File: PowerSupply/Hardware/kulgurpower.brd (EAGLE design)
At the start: 102 x 86.5 mm, 138 parts, among them M1 MST2V, M2 MST2V, M3 MST2V, M4 MST2V, X1 1727036, X2 2534-, X3 22-23-2031, X4 22-23-2031, X5 22-23-2021

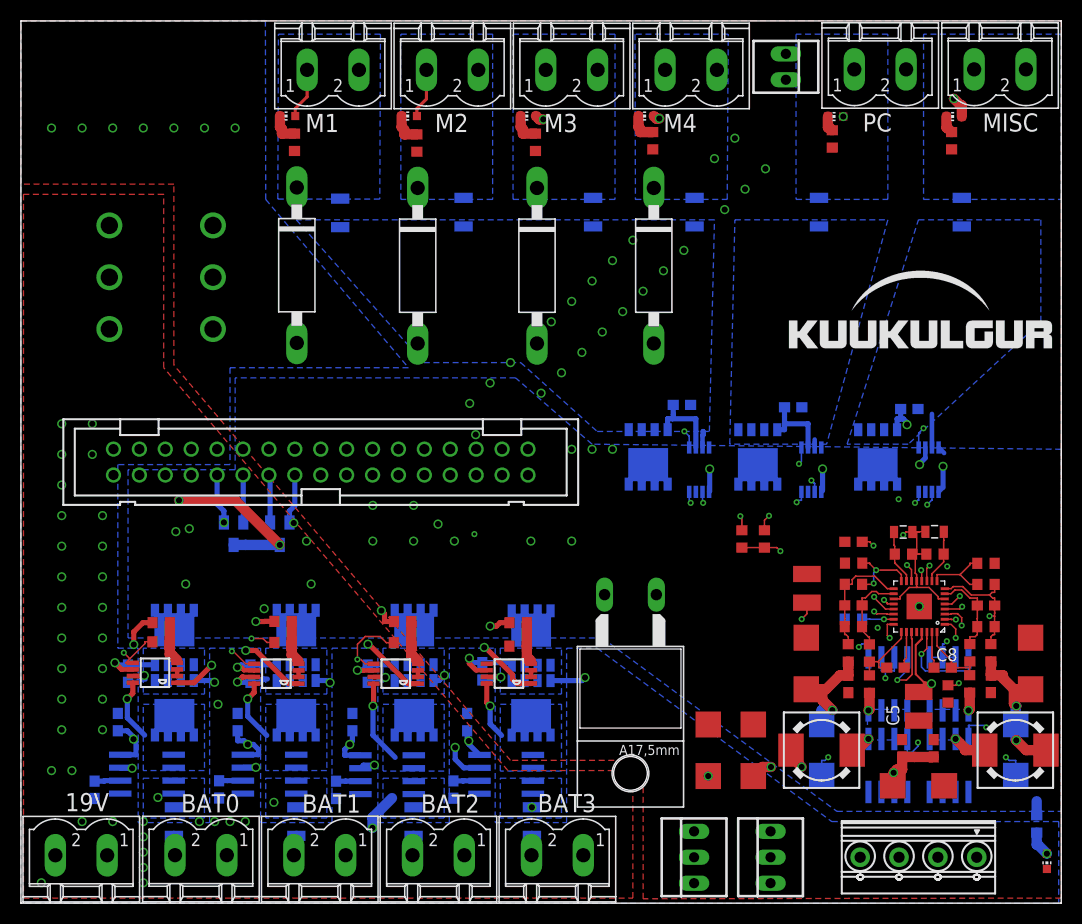
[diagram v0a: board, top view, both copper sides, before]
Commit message: Minor fixes to PCB
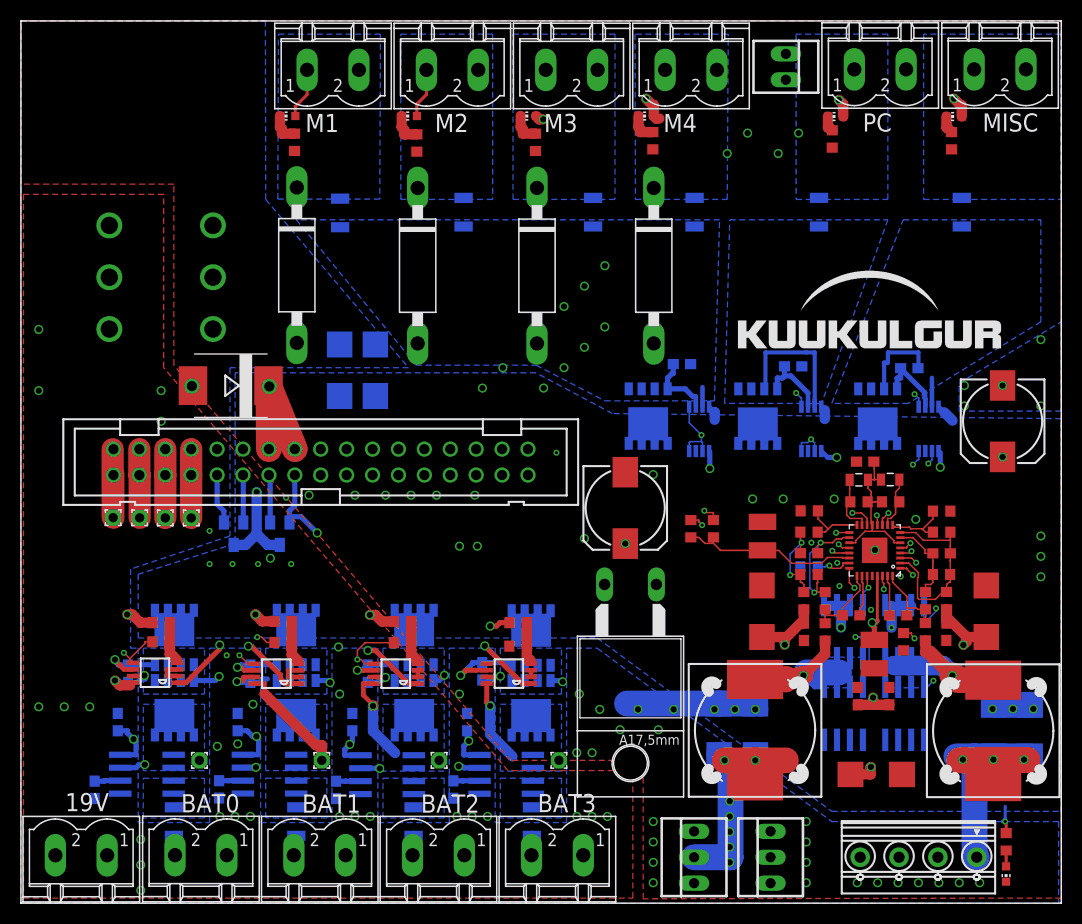
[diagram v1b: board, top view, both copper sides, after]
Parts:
- removed C13, C14: (no value), rcl:C/6032-28R
- added C31, C35: (no value), rcl:C/6032-28R
- added C36, C37: 15V, rcl:C/6032-28R
- added C38: 15V, rcl:175TMP-0810
- added C39: 15v, rcl:175TMP-0810
- added D4: MBRS330T3, diode:SMC
- added PAD1, PAD2, PAD3, PAD4, PAD5, PAD6, PAD7, PAD8: (no value), wirepad:1,6/0,9
- C104, C113, C32: value 220n -> 0.1
- C3: value (none) -> 15V
- L1, L2: device inductors:DR73 -> inductors:DR125
- moved C10 7.95 mm to (82.8, 43.3)
- moved U$17 7.02 mm to (83.7, 34.6)
- moved L2 6.81 mm to (72.0, 17.0), turned to 270 degrees
- moved SJ104 6.72 mm to (77.3, 33.0)
- moved C1 6.72 mm to (94.6, 28.6)
- moved C16 6.72 mm to (90.3, 34.3)
- moved C17 6.72 mm to (72.7, 36.0)
- moved C2 6.72 mm to (72.6, 28.6)
- moved C20 6.72 mm to (77.3, 34.3)
- moved C21 6.72 mm to (81.4, 28.2)
- moved C29 6.72 mm to (85.1, 20.3)
- moved C33 6.72 mm to (82.2, 41.5)
- moved C5 6.72 mm to (83.7, 24.4)
- moved R21 6.72 mm to (90.3, 36.4)
- moved R23 6.72 mm to (85.3, 39.3)
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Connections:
- net 5V renamed 5V_LDO
- new net +19V_CHG: D4.C, X2.14, X2.16
- new net N$2: D4.A
- net +19V: no longer X2.14, X2.16
- net +5V: now also C31.+, C35.+; no longer C13.+
- net GND: now also C31.-, C35.-, C36.-, C37.-, C38.-, C39.-; no longer C13.-, C14.-
- net SERVO: no longer C14.+
- net V+: now also C36.+, C37.+, C38.+, C39.+
- net VBAT0: no longer X2.1, X2.2
- net VBAT0_X: now also PAD1.1, PAD8.1, X2.1, X2.2
- net VBAT1: no longer X2.3, X2.4
- net VBAT1_X: now also PAD2.1, PAD7.1, X2.3, X2.4
- net VBAT2: no longer X2.5, X2.6
- net VBAT2_X: now also PAD3.1, PAD6.1, X2.5, X2.6
- net VBAT3: no longer X2.7, X2.8
- net VBAT3_X: now also PAD4.1, PAD5.1, X2.7, X2.8
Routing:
- net VBAT3: track 61.2 -> 0.00 mm, vias 2 -> 0
- net VBAT2: track 53.1 -> 0.00 mm, vias 3 -> 0
- net VBAT3_X: track 15.8 -> 60.0 mm
- net VBAT1_X: track 16.1 -> 58.7 mm
- net VBAT1: track 40.1 -> 0.00 mm, vias 2 -> 0
- net VBAT0: track 40.0 -> 0.00 mm, vias 1 -> 0
- net VBAT0_X: track 15.1 -> 47.5 mm
- net VBAT2_X: track 20.0 -> 52.1 mm
- net +5V: track 27.6 -> 55.5 mm, vias 2 -> 4
- net SERVO: track 16.9 -> 39.6 mm, vias 4 -> 8
- net GND: track 47.1 -> 64.6 mm, vias 60 -> 92
- net X2: track 3.82 -> 18.3 mm, vias 2 -> 1
- net X1: track 5.22 -> 19.6 mm, vias 2 -> 1
- net OUT2_S: track 0.79 -> 13.8 mm
- net +19V_CHG: track 0.00 -> 13.0 mm, vias 0 -> 1
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- added copper zone on layer 15, net +5V
